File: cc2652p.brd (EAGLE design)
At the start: 25.3 x 57.3 mm, 51 parts, among them IC2 CP2102, J3 CORTEX_DEBUG_SMD, J5 TYPE-C-31-M-12, Q1 SI2323DS, Q2 SI2323DS, U1 MCP73831, U2 ap2112k-3.3, U3 XC61CN3202MR-G, U4 MMDT2907A-7-F, U5 MX25R8035FZUIL0

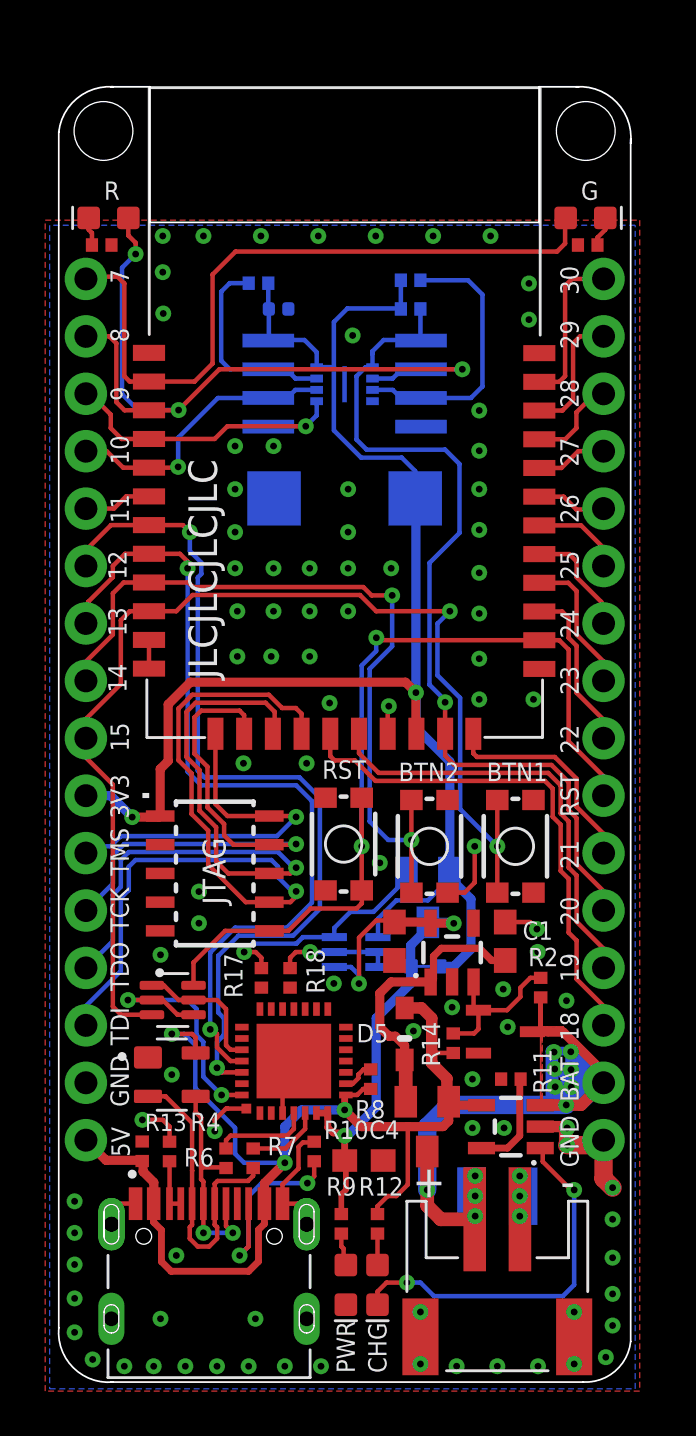
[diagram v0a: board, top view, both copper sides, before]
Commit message: Add files via upload
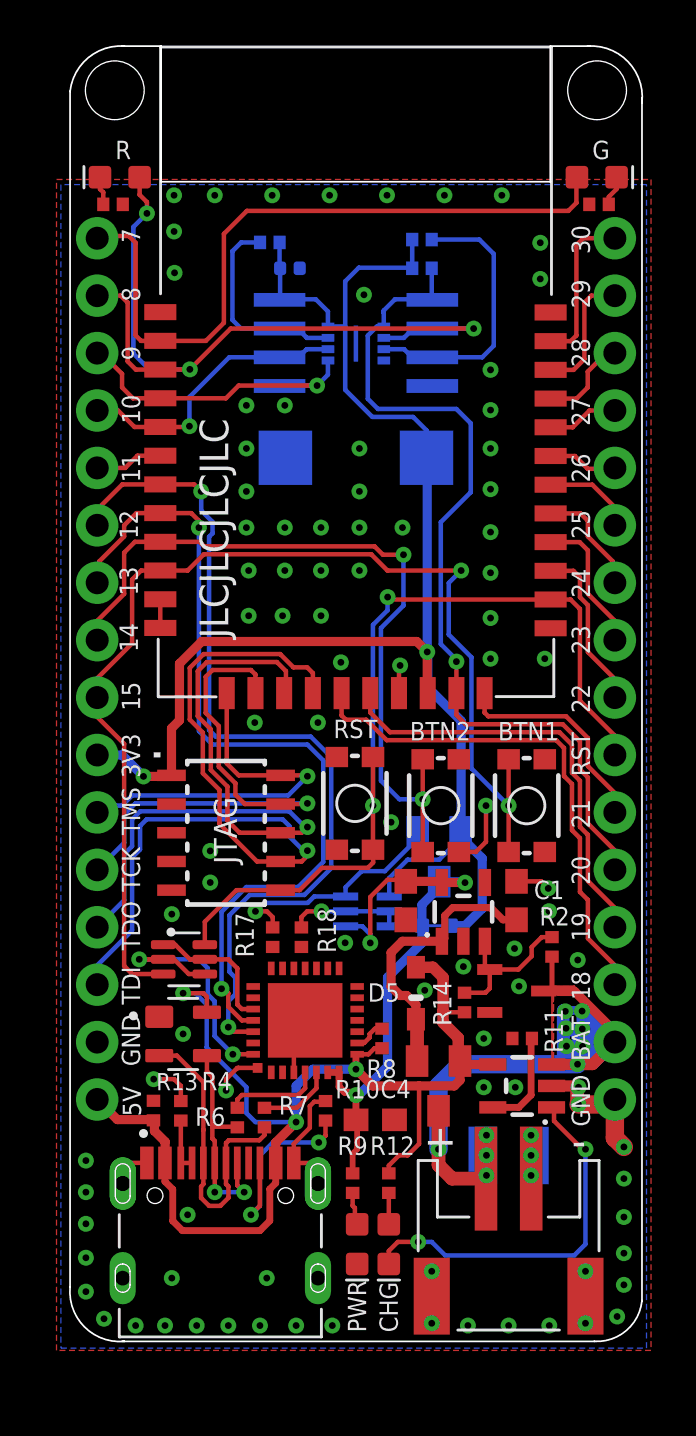
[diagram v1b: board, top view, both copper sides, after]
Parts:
- R1: value 2.2k -> 100k
- R15, R16: value 0 -> 10k
- U5: value MX25R8035FZUIL0 -> W25X40CL
- moved C13 1.87 mm to (12.6, 39.3)
- moved D1 1.87 mm to (2.13, 51.7)
- moved D2 1.87 mm to (23.2, 51.7)
- moved R16 1.87 mm to (15.5, 48.9)
- moved BTN1 1.87 mm to (20.1, 23.9)
- moved BTN2 1.87 mm to (16.3, 23.9)
- moved D4 1.87 mm to (4.93, 13.8)
- moved D5 1.87 mm to (15.2, 15.6)
- moved R11 1.87 mm to (19.9, 13.6)
- moved R14 1.87 mm to (17.4, 15.2)
- moved R17 1.87 mm to (8.89, 18.1)
- moved R18 1.87 mm to (10.2, 18.1)
- moved R2 1.87 mm to (21.2, 17.7)
- moved R6 1.87 mm to (7.33, 10.1)
- moved R7 1.87 mm to (8.53, 10.1)
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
